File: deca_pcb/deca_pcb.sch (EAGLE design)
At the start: 8 parts, among them IC1 DWM1000, IC2 LM340H-18, U1 ATMEGA328P-PU, X1 MINI-USB-32005-301, X2 332-06

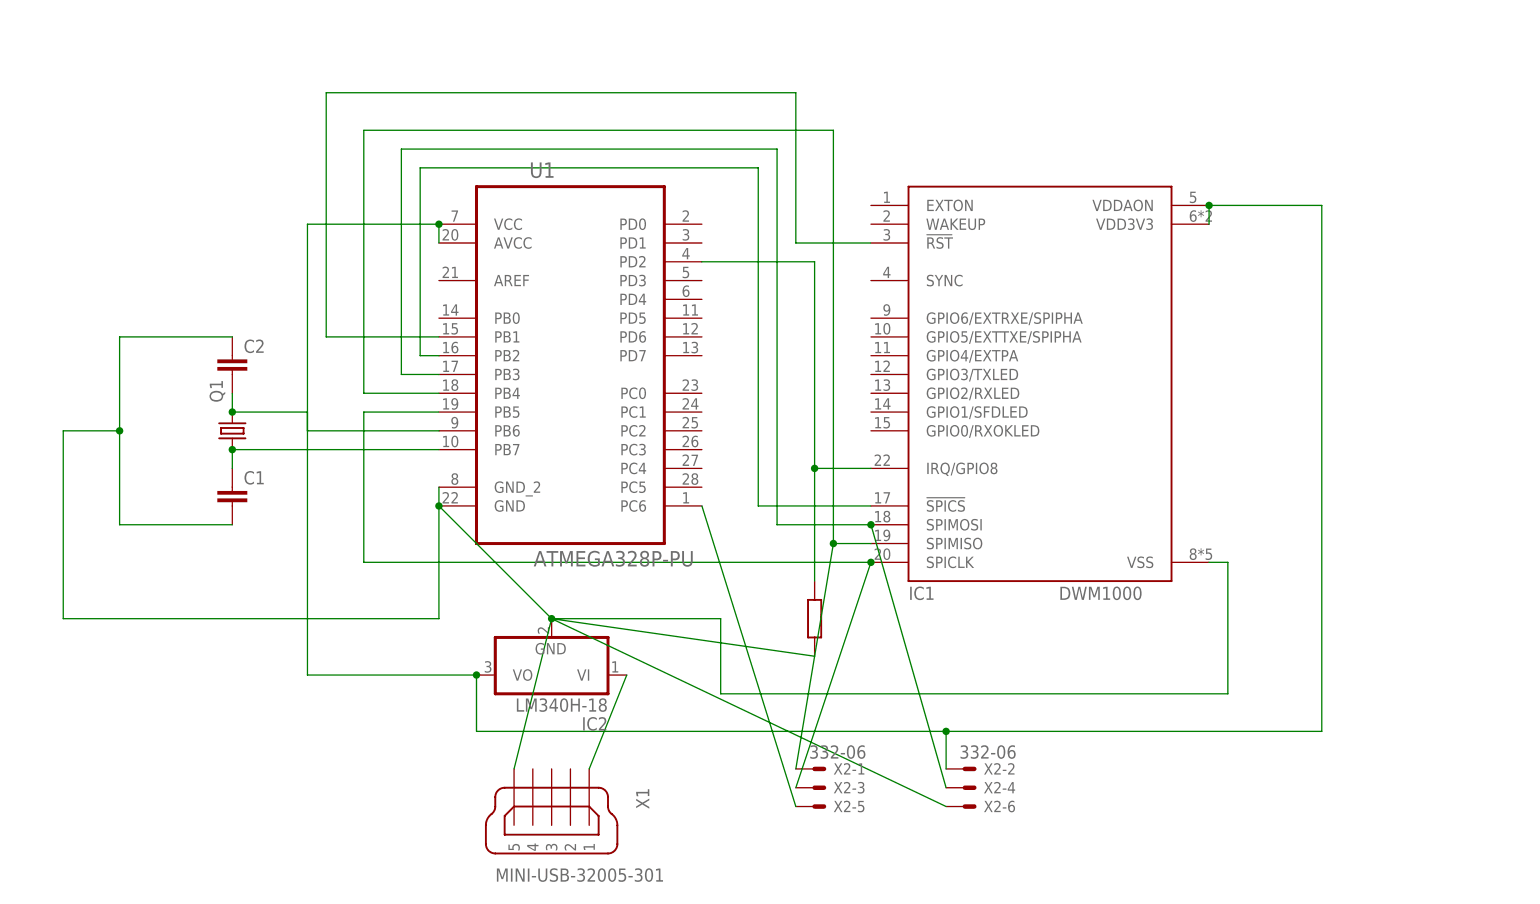
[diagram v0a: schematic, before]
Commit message: board pcb done
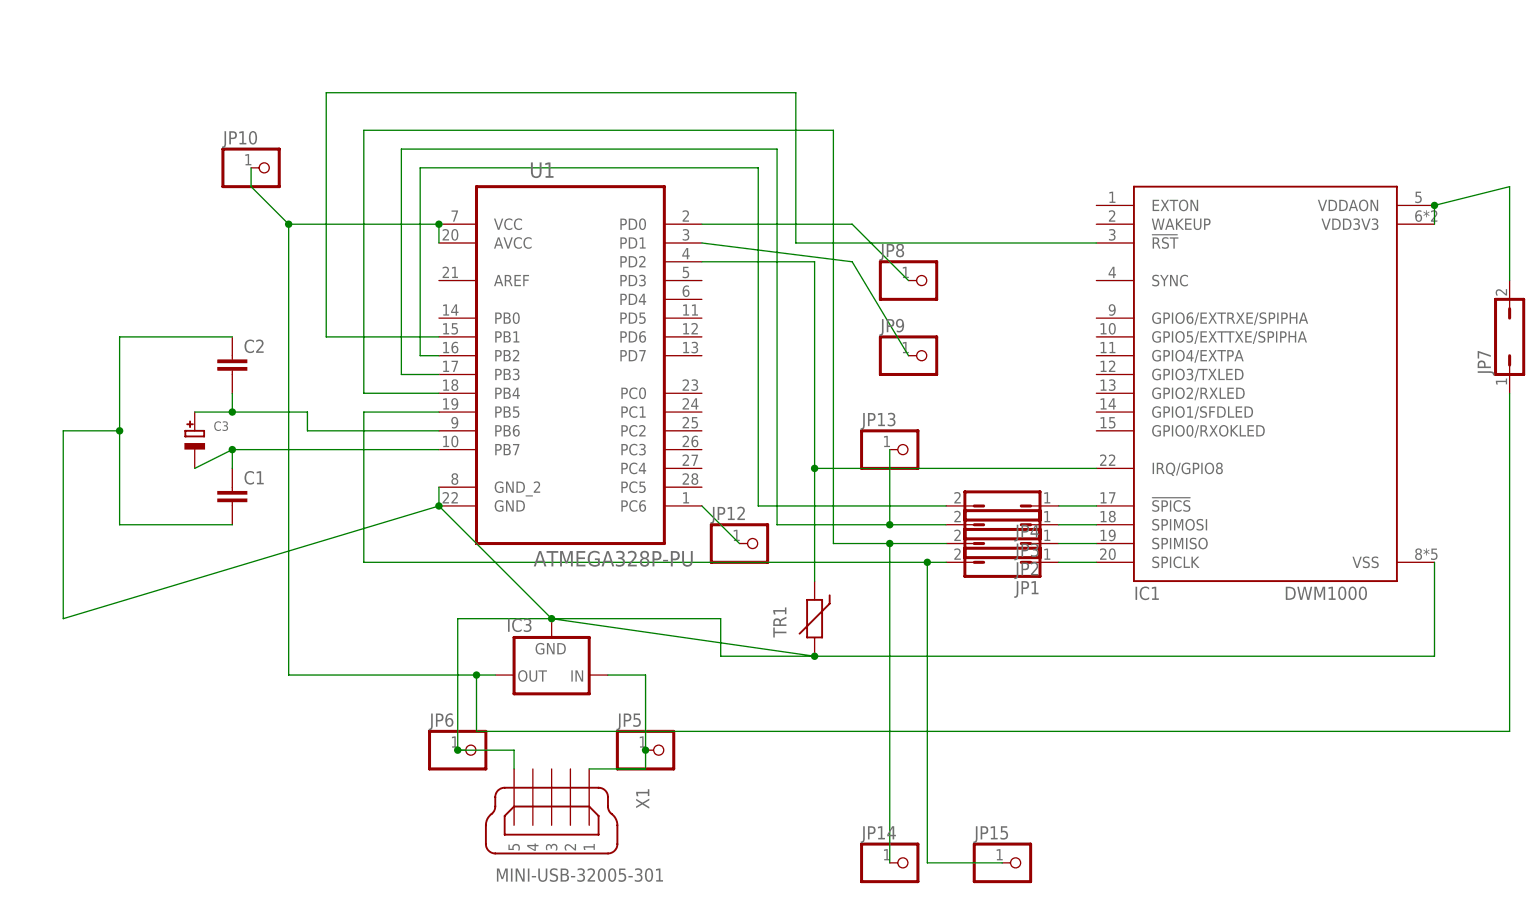
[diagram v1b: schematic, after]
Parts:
- removed IC2: LM340H-18, linear:LM340H-18
- removed Q1: (no value), crystal-geyer_V1_0:KX-9B
- removed X2: 332-06, con-garry:332-06
- added C3: (no value), microbuilder:CAP_ELECTROLYTICPTH_3.5MMGRID_8MMDIA
- added IC3: (no value), lf33:LFXXCVS
- added JP1, JP2, JP3, JP4, JP7: (no value), jumper:JP1Q
- added JP10, JP12, JP13, JP14, JP15, JP5, JP6, JP8, JP9: (no value), con-pinhead:PINHD-1X1_2.54
- added TR1: (no value), discrete:THERMISTOR_R-5
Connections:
- new net N$13: C1.2, C2.1, IC1.VSS, IC3.GND, JP6.1, TR1.2, U1.GND, U1.GND_2, X1.5
- new net N$14: IC1.SPIMISO, JP2.1
- new net N$15: IC1.SPIMOSI, JP3.1
- new net N$16: IC1.!SPICS, JP4.1
- new net N$17: JP8.1, U1.PD0
- new net N$18: JP9.1, U1.PD1
- new net N$19: JP12.1, U1.PC6
- net N$1: now also JP1.2, JP15.1; no longer IC1.SPICLK, X2-3.S
- net N$10: now also IC3.IN, JP5.1; no longer IC2.VI
- net N$11: now also IC1.SPICLK, JP1.1; no longer C1.2, C2.1, IC1.VSS, IC2.GND, U1.GND, U1.GND_2, X1.5, X2-6.S
- net N$12: now also IC3.OUT, JP10.1, JP7.1; no longer IC1.VDD3V3, IC1.VDDAON, IC2.VO, X2-2.S
- net N$2: now also JP14.1, JP2.2; no longer IC1.SPIMISO, X2-1.S
- net N$3: now also JP13.1, JP3.2; no longer IC1.SPIMOSI, X2-4.S
- net N$4: now also JP4.2; no longer IC1.!SPICS
- net N$5: now also TR1.1
- net N$7: now also C3.+; no longer Q1.2
- net N$8: now also C3.-; no longer Q1.1
- net N$9: now also IC1.VDD3V3, IC1.VDDAON, JP7.2; no longer U1.PC6, X2-5.S
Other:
- moved on the sheet: IC1

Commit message: txt
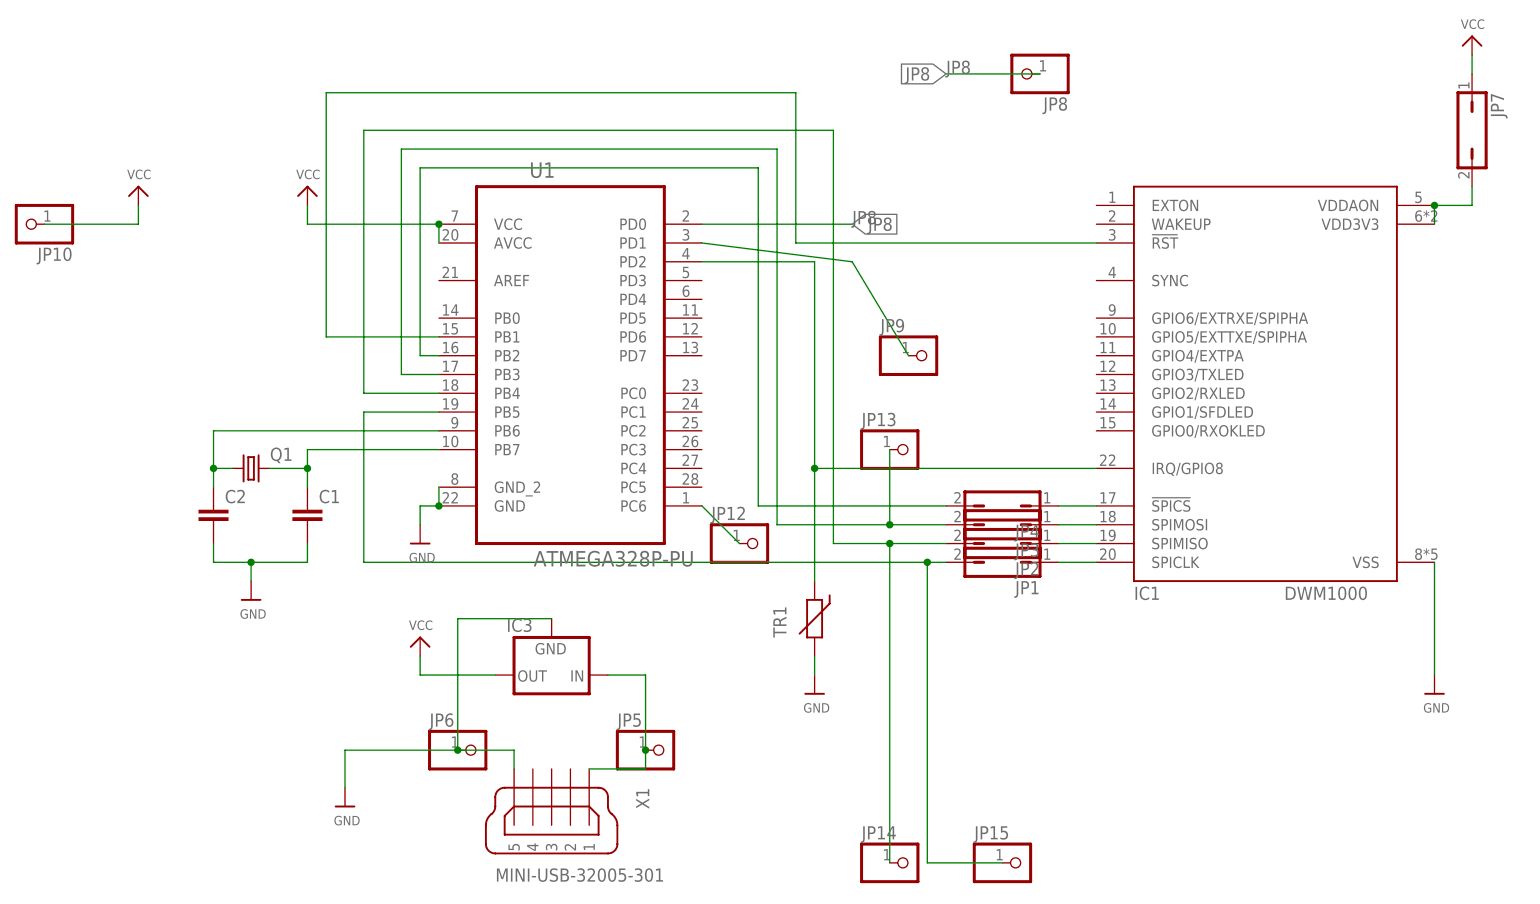
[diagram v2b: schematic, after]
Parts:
- removed C3: (no value), microbuilder:CAP_ELECTROLYTICPTH_3.5MMGRID_8MMDIA
- added Q1: (no value), crystal:CRYSTALHC49S
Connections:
- net N$12 renamed VCC
- net N$17 renamed JP8
- removed net N$13: C1.2, C2.1, IC1.VSS, IC3.GND, JP6.1, TR1.2, U1.GND, U1.GND_2, X1.5
- new net GND: C1.2, C2.2, IC1.VSS, IC3.GND, JP6.1, TR1.2, U1.GND, U1.GND_2, X1.5
- net N$7: now also C2.1, Q1.1; no longer C2.2, C3.+
- net N$8: now also Q1.2; no longer C3.-
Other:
- moved on the sheet: C1, C2, JP10, JP7, JP8
